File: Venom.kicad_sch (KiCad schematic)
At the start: 14 parts, among them CN1 HC-XH-5A-G, CN2 HC-PH-8A-G, CN3 HC-XH-8A-G, CN4 HC-XH-8A-G, CN5 HC-XH-2A-G, CN6 HC-PH-7A-G, SW1 GT-TC030A-H020-L1N, SW2 GT-TC030A-H020-L1N, U1 Pico

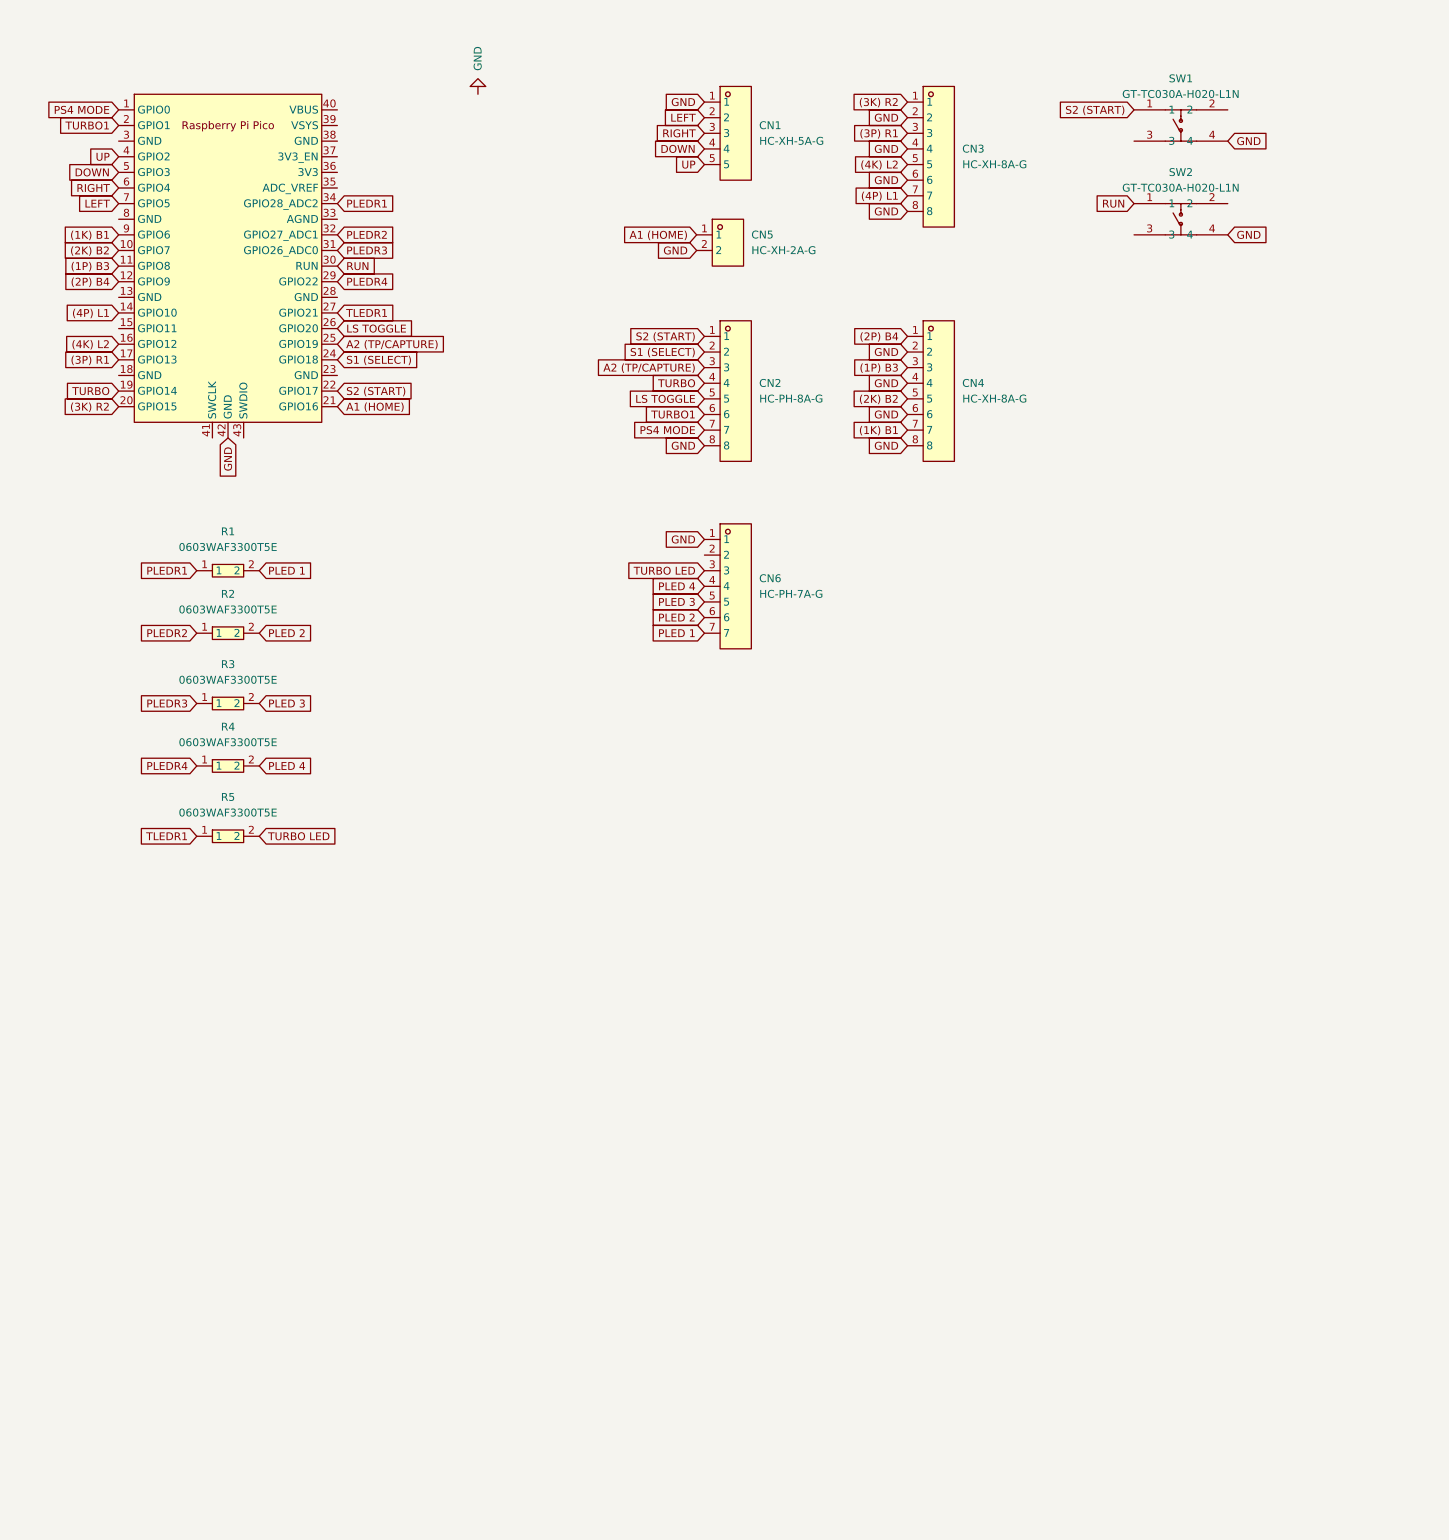
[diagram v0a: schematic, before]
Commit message: WIP embedded design
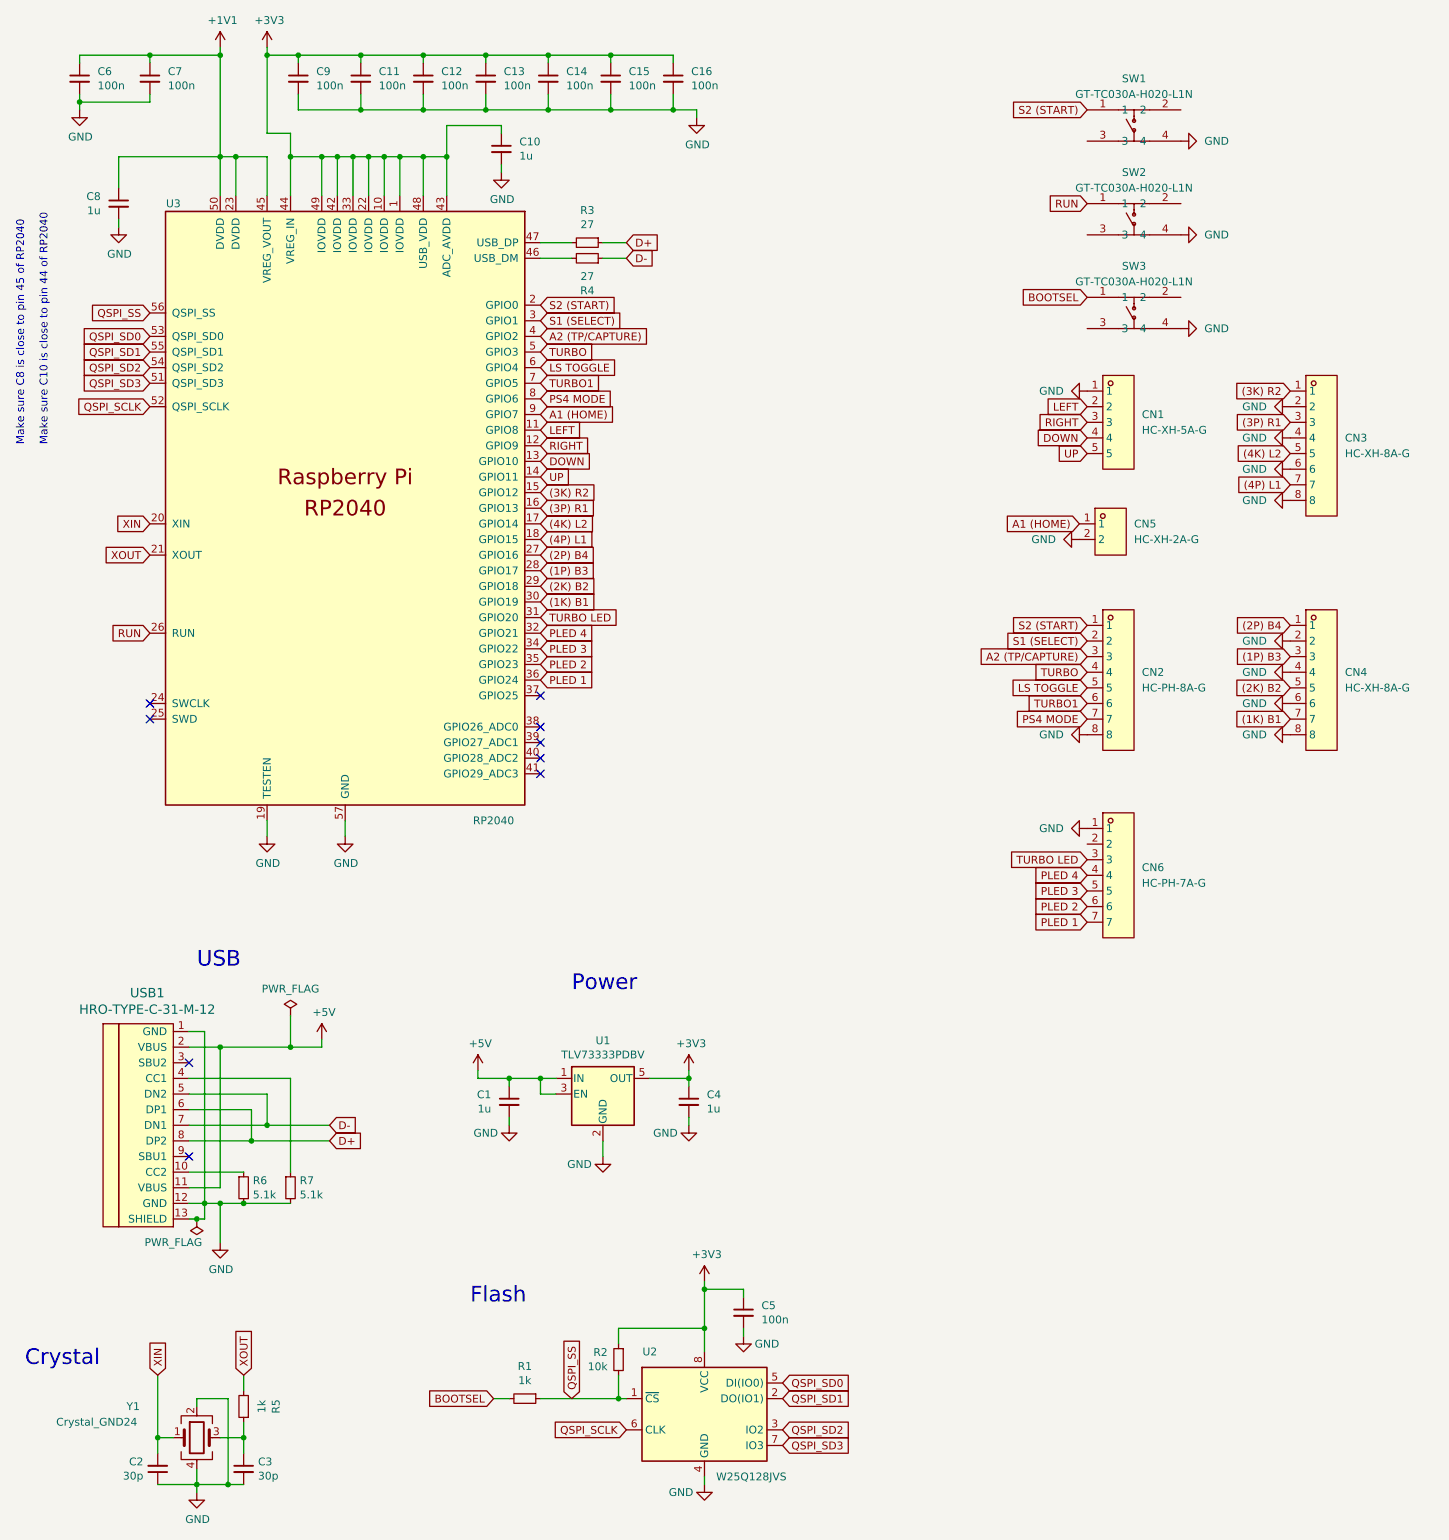
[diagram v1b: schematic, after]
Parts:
- removed R1, R2, R3, R4, R5: 0603WAF3300T5E, easyeda2kicad:R0603, symbol easyeda2kicad:0603WAF3300T5E
- removed U1: Pico, MCU_RaspberryPi_and_Boards:RPi_Pico_SMD_TH, symbol MCU_RaspberryPi_and_Boards:Pico
- added C1, C10, C4, C8: 1u, Capacitor_SMD:C_0402_1005Metric, symbol Device:C_Small
- added C11, C12, C13, C14, C15, C16, C5, C6, C7, C9: 100n, Capacitor_SMD:C_0402_1005Metric, symbol Device:C_Small
- added C2, C3: 30p, Capacitor_SMD:C_0402_1005Metric, symbol Device:C_Small
- added R1, R5: 1k, Resistor_SMD:R_0402_1005Metric, symbol Device:R_Small
- added R2: 10k, Resistor_SMD:R_0402_1005Metric, symbol Device:R_Small
- added R3, R4: 27, Resistor_SMD:R_0402_1005Metric, symbol Device:R_Small
- added R6, R7: 5.1k, Resistor_SMD:R_0402_1005Metric, symbol Device:R_Small
- added SW3: GT-TC030A-H020-L1N, easyeda2kicad:SW-SMD_4P-L3.6-W3.0-P1.50-LS4.7, symbol easyeda2kicad:GT-TC030A-H020-L1N
- added U1: TLV73333PDBV, Package_TO_SOT_SMD:SOT-23-5, symbol Regulator_Linear:TLV73333PDBV
- added U2: W25Q128JVS, Package_SO:SOIC-8_5.23x5.23mm_P1.27mm, symbol Flatbox-rev4-rescue:W25Q128JVS-Memory_Flash
- added U3: RP2040, RP2040:RP2040-QFN-56, symbol RP2040:RP2040
- added USB1: HRO-TYPE-C-31-M-12, Type-C:HRO-TYPE-C-31-M-12-Assembly, symbol Type-C:HRO-TYPE-C-31-M-12
- added Y1: Crystal_GND24, Crystal:Crystal_SMD_3225-4Pin_3.2x2.5mm, symbol Device:Crystal_GND24
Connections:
- net (1K) B1: now also U3.30 (GPIO19)
- net (1P) B3: now also U3.28 (GPIO17)
- net (2K) B2: now also U3.29 (GPIO18)
- net (2P) B4: now also U3.27 (GPIO16)
- net (3K) R2: now also U3.15 (GPIO12)
- net (3P) R1: now also U3.16 (GPIO13)
- net (4K) L2: now also U3.17 (GPIO14)
- net (4P) L1: now also U3.18 (GPIO15)
- net A1 (HOME): now also U3.9 (GPIO7)
- net A2 (TP/CAPTURE): now also U3.4 (GPIO2)
- net DOWN: now also U3.13 (GPIO10)
- net GND: now also C1.2, C10.2, C11.2, C12.2, C13.2, C14.2, C15.2, C16.2, C2.1, C3.2, C4.2, C5.2, C6.2, C7.2, C8.2, C9.2, R6.2, R7.2, SW3.4, U1.2 (GND), U2.4 (GND), U3.19 (TESTEN), U3.57 (GND), USB1.1 (GND), USB1.12 (GND), USB1.13 (SHIELD), Y1.2, Y1.4
- net LEFT: now also U3.11 (GPIO8)
- net LS TOGGLE: now also U3.6 (GPIO4)
- net PLED 1: now also U3.36 (GPIO24)
- net PLED 2: now also U3.35 (GPIO23)
- net PLED 3: now also U3.34 (GPIO22)
- net PLED 4: now also U3.32 (GPIO21)
- net PS4 MODE: now also U3.8 (GPIO6)
- net RIGHT: now also U3.12 (GPIO9)
- net RUN: now also U3.26 (RUN)
- net S1 (SELECT): now also U3.3 (GPIO1)
- net S2 (START): now also U3.2 (GPIO0)
- net TURBO: now also U3.5 (GPIO3)
- net TURBO LED: now also U3.31 (GPIO20)
- net TURBO1: now also U3.7 (GPIO5)
- net UP: now also U3.14 (GPIO11)
- new net: R7.1, USB1.4 (CC1)
- new net: R6.1, USB1.10 (CC2)
- new net: C3.1, R5.1, Y1.3
- new net: R4.2, U3.46 (USB_DM)
- new net: R3.2, U3.47 (USB_DP)
- new net +1V1: C6.1, C7.1, C8.1, U3.23 (DVDD), U3.45 (VREG_VOUT), U3.50 (DVDD)
- new net +3V3: C10.1, C11.1, C12.1, C13.1, C14.1, C15.1, C16.1, C4.1, C5.1, C9.1, R2.1, U1.5 (OUT), U2.8 (VCC), U3.1 (IOVDD), U3.10 (IOVDD), U3.22 (IOVDD), U3.33 (IOVDD), U3.42 (IOVDD), U3.43 (ADC_AVDD), U3.44 (VREG_IN), U3.48 (USB_VDD), U3.49 (IOVDD)
- new net +5V: C1.1, U1.1 (IN), U1.3 (EN), USB1.11 (VBUS), USB1.2 (VBUS)
- new net BOOTSEL: R1.2, SW3.1
- new net D+: R3.1, USB1.6 (DP1), USB1.8 (DP2)
- new net D-: R4.1, USB1.5 (DN2), USB1.7 (DN1)
- new net QSPI_SCLK: U2.6 (CLK), U3.52 (QSPI_SCLK)
- new net QSPI_SD0: U2.5 (DI(IO0)), U3.53 (QSPI_SD0)
- new net QSPI_SD1: U2.2 (DO(IO1)), U3.55 (QSPI_SD1)
- new net QSPI_SD2: U2.3 (IO2), U3.54 (QSPI_SD2)
- new net QSPI_SD3: U2.7 (IO3), U3.51 (QSPI_SD3)
- new net QSPI_SS: R1.1, R2.2, U2.1 (~{CS}), U3.56 (QSPI_SS)
- new net XIN: C2.2, U3.20 (XIN), Y1.1
- new net XOUT: R5.2, U3.21 (XOUT)
- no-connect marks 0 -> 9
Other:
- note added: "Crystal"
- note added: "Flash"
- note added: "Make sure C10 is close to pin 44 of RP2040"
- note added: "Make sure C8 is close to pin 45 of RP2040"
- note added: "Power"
- note added: "USB"
- moved on the sheet: CN1, CN2, CN3, CN4, CN5, CN6, SW1, SW2
